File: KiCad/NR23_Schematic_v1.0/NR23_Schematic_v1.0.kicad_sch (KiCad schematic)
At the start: 0 parts

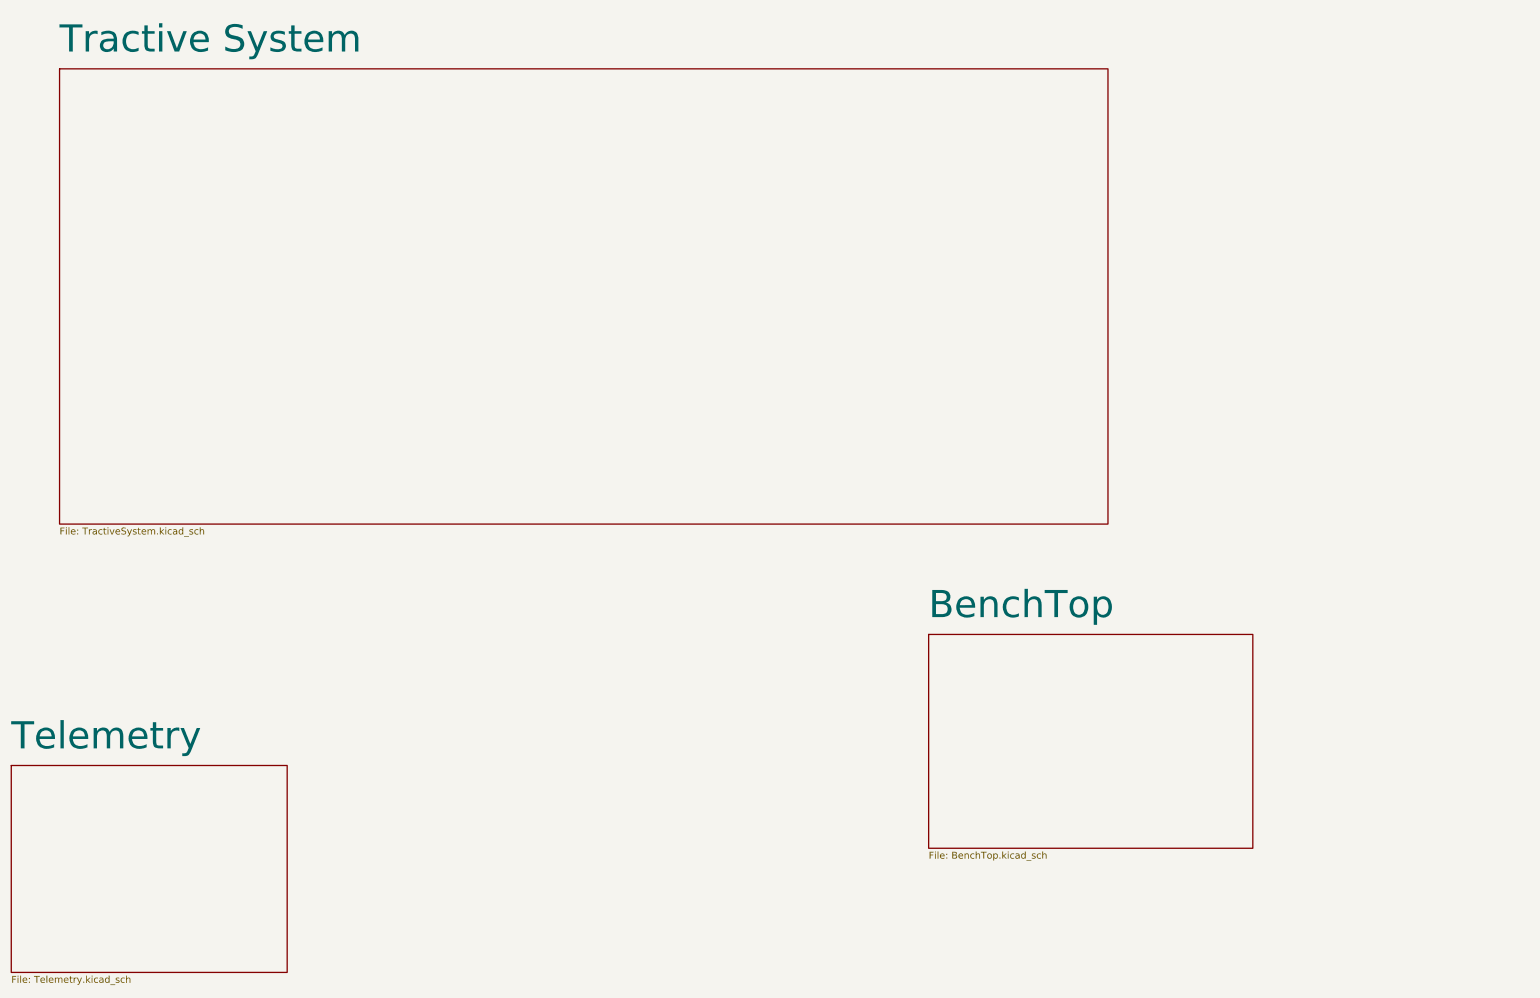
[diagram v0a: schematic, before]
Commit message: start of class 18APR23
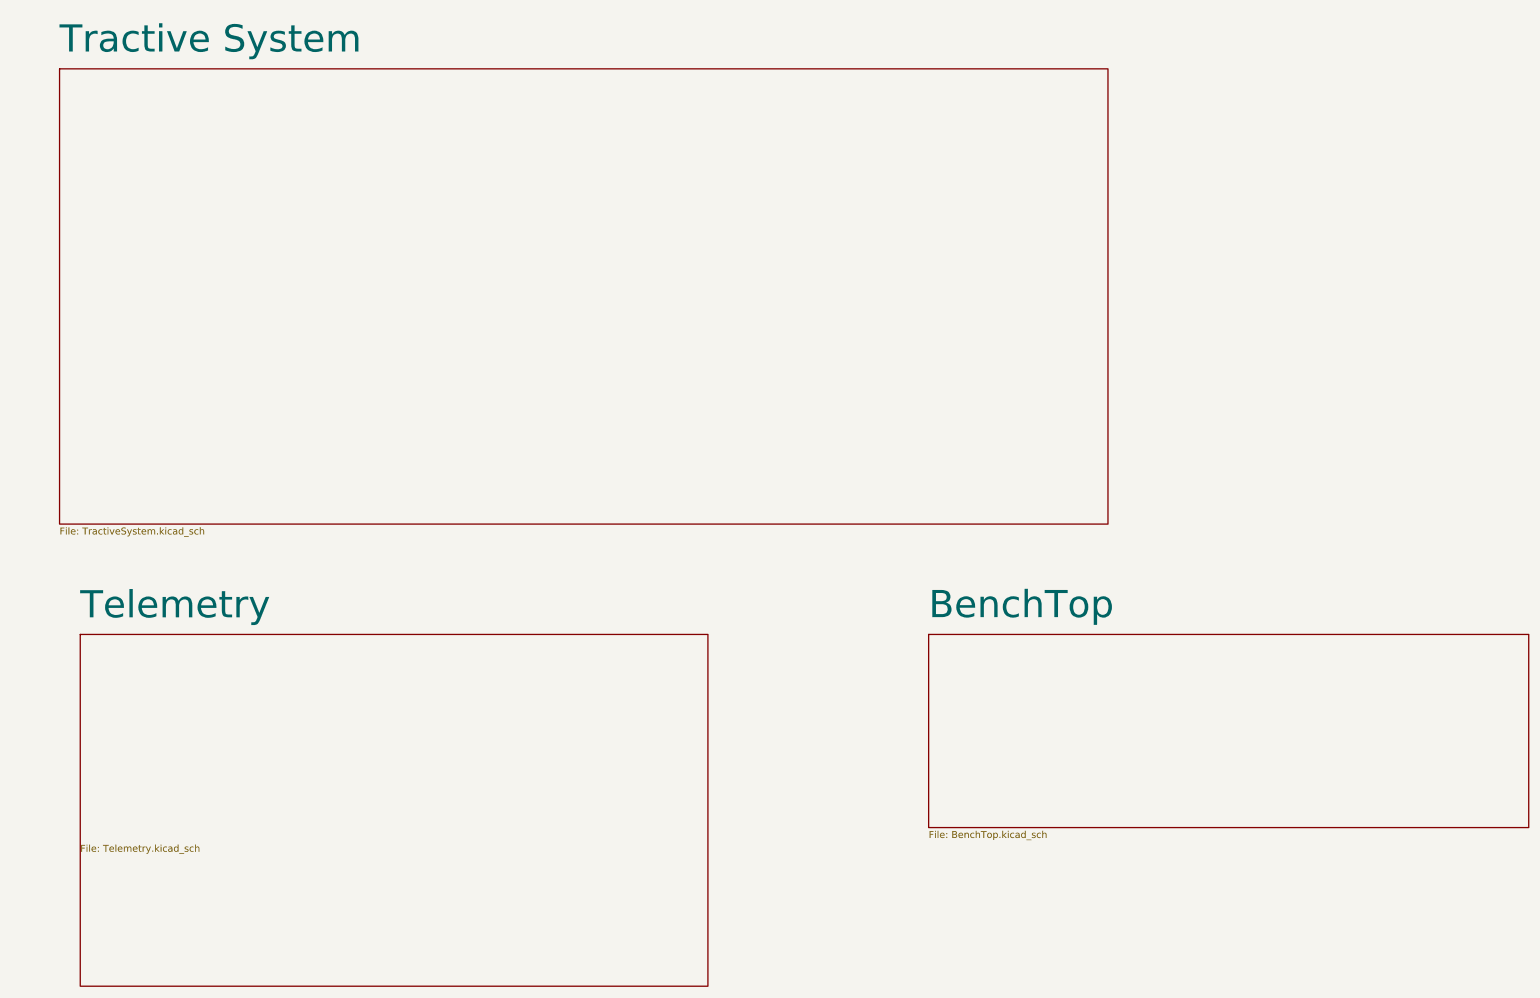
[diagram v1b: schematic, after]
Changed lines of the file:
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@@
     (date "2023-04-04")
   )
-  (sheet (at 26.67 156.21) (size 50.8 38.1)
+  (sheet (at 39.37 132.08) (size 115.57 64.77)
     (stroke (width 0.1524) (type solid) (color 0 0 0 0))
     (fill (color 0 0 0 0.0000))
-    (property "Sheet name" "Telemetry" (id 0) (at 26.67 153.67 0)
+    (property "Sheet name" "Telemetry" (id 0) (at 39.37 129.54 0)
       (effects (font (size 5 5)) (justify left bottom))
     )
-    (property "Sheet file" "Telemetry.kicad_sch" (id 1) (at 26.67 194.8946 0)
+    (property "Sheet file" "Telemetry.kicad_sch" (id 1) (at 39.37 170.7646 0)
       (effects (font (size 1.27 1.27)) (justify left top))
     )
   )
-  (sheet (at 195.58 132.08) (size 59.69 39.37) (fields_autoplaced)
+  (sheet (at 195.58 132.08) (size 110.49 35.56) (fields_autoplaced)
     (stroke (width 0.1524) (type solid) (color 0 0 0 0))
     (fill (color 0 0 0 0.0000))
@@
       (effects (font (size 5 5)) (justify left bottom))
     )
-    (property "Sheet file" "BenchTop.kicad_sch" (id 1) (at 195.58 172.0346 0)
+    (property "Sheet file" "BenchTop.kicad_sch" (id 1) (at 195.58 168.2246 0)
       (effects (font (size 1.27 1.27)) (justify left top))
     )
@@
   )
   (symbol_instances
+    (path "/8302703f-65d0-4b91-aeea-6f721ab57e4c/97abb871-5579-4630-a10b-2cee2773b5bb/0cc246a4-8870-49dd-945c-fbfffb55b703"
+      (reference "#PWR?") (unit 1) (value "GND") (footprint "")
+    )
+    (path "/8302703f-65d0-4b91-aeea-6f721ab57e4c/97abb871-5579-4630-a10b-2cee2773b5bb/5b678e11-7d21-49c7-87bd-7953081d7748"
+      (reference "#PWR?") (unit 1) (value "GND") (footprint "")
+    )
+    (path "/8302703f-65d0-4b91-aeea-6f721ab57e4c/97abb871-5579-4630-a10b-2cee2773b5bb/86242390-ce71-4a1c-a74a-66c29943dff8"
+      (reference "#PWR?") (unit 1) (value "GND") (footprint "")
+    )
+    (path "/8302703f-65d0-4b91-aeea-6f721ab57e4c/97abb871-5579-4630-a10b-2cee2773b5bb/934055cb-9d39-4ad1-ae76-261d73ee61b7"
+      (reference "#PWR?") (unit 1) (value "GND") (footprint "")
+    )
+    (path "/8302703f-65d0-4b91-aeea-6f721ab57e4c/97abb871-5579-4630-a10b-2cee2773b5bb/a095cb59-e422-4afa-939f-01dc6aa5dd91"
+      (reference "#PWR?") (unit 1) (value "GND") (footprint "")
+    )
     (path "/8302703f-65d0-4b91-aeea-6f721ab57e4c/97abb871-5579-4630-a10b-2cee2773b5bb/abd2a7f6-194b-4f90-9352-cc86eaabf27b"
       (reference "#PWR?") (unit 1) (value "GND") (footprint "")
     )
     (path "/8302703f-65d0-4b91-aeea-6f721ab57e4c/97abb871-5579-4630-a10b-2cee2773b5bb/aefa985d-2a08-4349-90af-e8fd54a309c3"
+      (reference "#PWR?") (unit 1) (value "GND") (footprint "")
+    )
+    (path "/8302703f-65d0-4b91-aeea-6f721ab57e4c/97abb871-5579-4630-a10b-2cee2773b5bb/b105d02e-5b3f-492d-b9d6-bccabd476c30"
       (reference "#PWR?") (unit 1) (value "GND") (footprint "")
     )
@@
       (reference "BTmain") (unit 1) (value "7.2KW_BatteryALLPINS") (footprint "")
     )
+    (path "/8302703f-65d0-4b91-aeea-6f721ab57e4c/97abb871-5579-4630-a10b-2cee2773b5bb/33edf8a8-a3e4-48e9-80f7-6f14e9047a71"
+      (reference "D?") (unit 1) (value "D") (footprint "")
+    )
+    (path "/8302703f-65d0-4b91-aeea-6f721ab57e4c/97abb871-5579-4630-a10b-2cee2773b5bb/3dd41065-0661-4611-b751-7b7457dab073"
+      (reference "D?") (unit 1) (value "D") (footprint "")
+    )
+    (path "/8302703f-65d0-4b91-aeea-6f721ab57e4c/97abb871-5579-4630-a10b-2cee2773b5bb/cb3f31f3-7647-4909-937e-3d544217c1ef"
+      (reference "D?") (unit 1) (value "D") (footprint "")
+    )
     (path "/8302703f-65d0-4b91-aeea-6f721ab57e4c/0ff0a299-f28e-4254-8f91-d87a10b36f6c"
       (reference "F?") (unit 1) (value "Sevcon Fuse") (footprint "")
@@
       (reference "F?") (unit 1) (value "Fuse") (footprint "")
     )
+    (path "/8302703f-65d0-4b91-aeea-6f721ab57e4c/c3efaf65-8006-4868-9f6d-0b34664fb679"
+      (reference "HVSS") (unit 1) (value "HV Safety Switch (behind driver)") (footprint "")
+    )
     (path "/8302703f-65d0-4b91-aeea-6f721ab57e4c/97abb871-5579-4630-a10b-2cee2773b5bb/1dd5ea95-d588-470f-9d97-474e57890a75"
       (reference "J?") (unit 1) (value "Display Connection") (footprint "")
@@
       (reference "J?") (unit 1) (value "Dash Key Switch Connection") (footprint "")
     )
-    (path "/8302703f-65d0-4b91-aeea-6f721ab57e4c/4f7773d6-0ce1-4de2-b33c-40a7545a2a6c"
-      (reference "J?") (unit 1) (value "Dash 12 power connection") (footprint "")
-    )
     (path "/8302703f-65d0-4b91-aeea-6f721ab57e4c/677d3ecc-41bd-42e2-8c0e-9eee2eeadf6d"
       (reference "J?") (unit 1) (value "Alt Dash 12 power connection") (footprint "")
@@
       (reference "M1") (unit 1) (value "Zero_7R_Motor") (footprint "")
     )
+    (path "/8302703f-65d0-4b91-aeea-6f721ab57e4c/97abb871-5579-4630-a10b-2cee2773b5bb/4cfe98f9-aa78-4658-9e93-07cade6de232"
+      (reference "Q?") (unit 1) (value "Q_NMOS_DGS") (footprint "")
+    )
+    (path "/8302703f-65d0-4b91-aeea-6f721ab57e4c/97abb871-5579-4630-a10b-2cee2773b5bb/d68c45a5-3fdd-4a29-9ea0-4fa67786e0ef"
+      (reference "Q?") (unit 1) (value "Q_NMOS_DGS") (footprint "")
+    )
+    (path "/8302703f-65d0-4b91-aeea-6f721ab57e4c/97abb871-5579-4630-a10b-2cee2773b5bb/faf03bf7-4254-4b9f-b70e-e4b84b8615c6"
+      (reference "Q?") (unit 1) (value "Q_NMOS_DGS") (footprint "")
+    )
+    (path "/8302703f-65d0-4b91-aeea-6f721ab57e4c/97abb871-5579-4630-a10b-2cee2773b5bb/2d9cf3fe-accd-4c59-87b2-dbf79ebc59cd"
+      (reference "R?") (unit 1) (value "R_US") (footprint "")
+    )
+    (path "/8302703f-65d0-4b91-aeea-6f721ab57e4c/97abb871-5579-4630-a10b-2cee2773b5bb/610df3be-18c0-42b0-9161-50b370e0205d"
+      (reference "R?") (unit 1) (value "R_US") (footprint "")
+    )
+    (path "/8302703f-65d0-4b91-aeea-6f721ab57e4c/97abb871-5579-4630-a10b-2cee2773b5bb/6917848f-da8c-4c38-8fa7-5aa80b3bfb19"
+      (reference "R?") (unit 1) (value "R_US") (footprint "")
+    )
+    (path "/8302703f-65d0-4b91-aeea-6f721ab57e4c/97abb871-5579-4630-a10b-2cee2773b5bb/abdb6156-d278-4176-813d-88b3fac1714c"
+      (reference "R?") (unit 1) (value "R_US") (footprint "")
+    )
+    (path "/8302703f-65d0-4b91-aeea-6f721ab57e4c/97abb871-5579-4630-a10b-2cee2773b5bb/c074acdc-73b0-49e5-a95e-d94754a448e2"
+      (reference "R?") (unit 1) (value "R_US") (footprint "")
+    )
+    (path "/8302703f-65d0-4b91-aeea-6f721ab57e4c/97abb871-5579-4630-a10b-2cee2773b5bb/c63e61ff-1cf3-4748-b8bd-e010cc68eeca"
+      (reference "R?") (unit 1) (value "R_US") (footprint "")
+    )
     (path "/8302703f-65d0-4b91-aeea-6f721ab57e4c/3c4e7487-ab0a-423b-bce9-bfd53c73f666"
       (reference "SW?") (unit 1) (value "Key Switch") (footprint "")
@@
       (reference "SW?") (unit 1) (value "100V E-stop (Left)") (footprint "")
     )
-    (path "/8302703f-65d0-4b91-aeea-6f721ab57e4c/c3efaf65-8006-4868-9f6d-0b34664fb679"
-      (reference "SW?") (unit 1) (value "HV Safety Switch (behind driver)") (footprint "")
-    )
     (path "/8302703f-65d0-4b91-aeea-6f721ab57e4c/c61cd80c-144e-4e2a-b98d-2afd10895cc1"
